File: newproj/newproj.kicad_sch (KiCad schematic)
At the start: 1 part

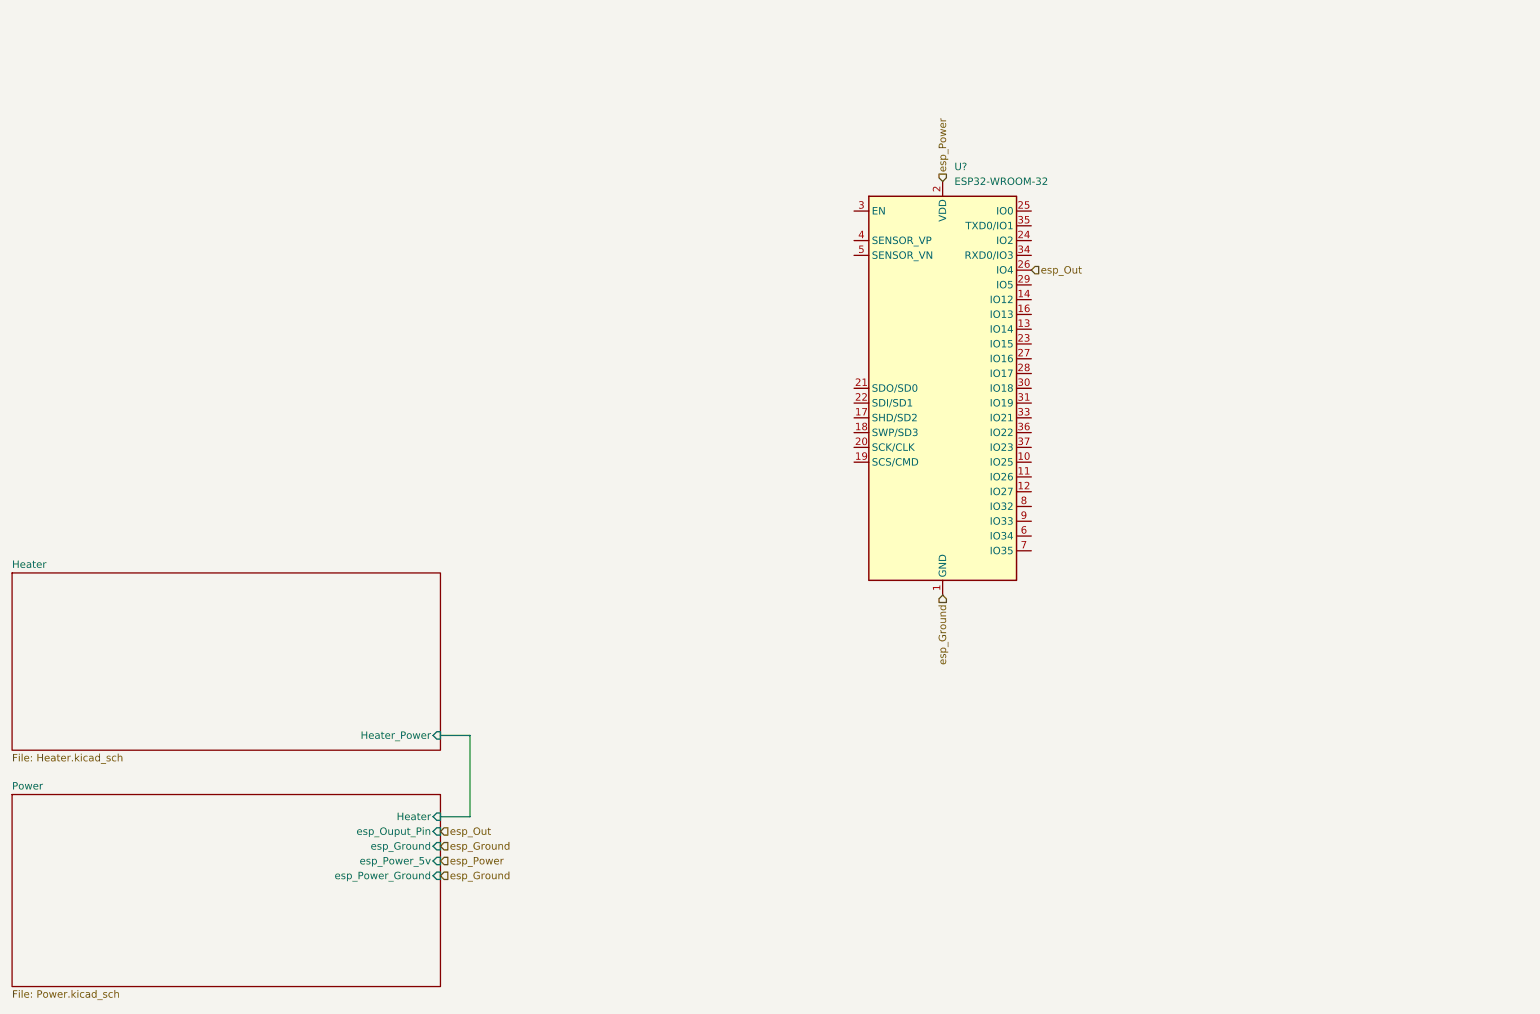
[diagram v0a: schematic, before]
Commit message: Add files via upload
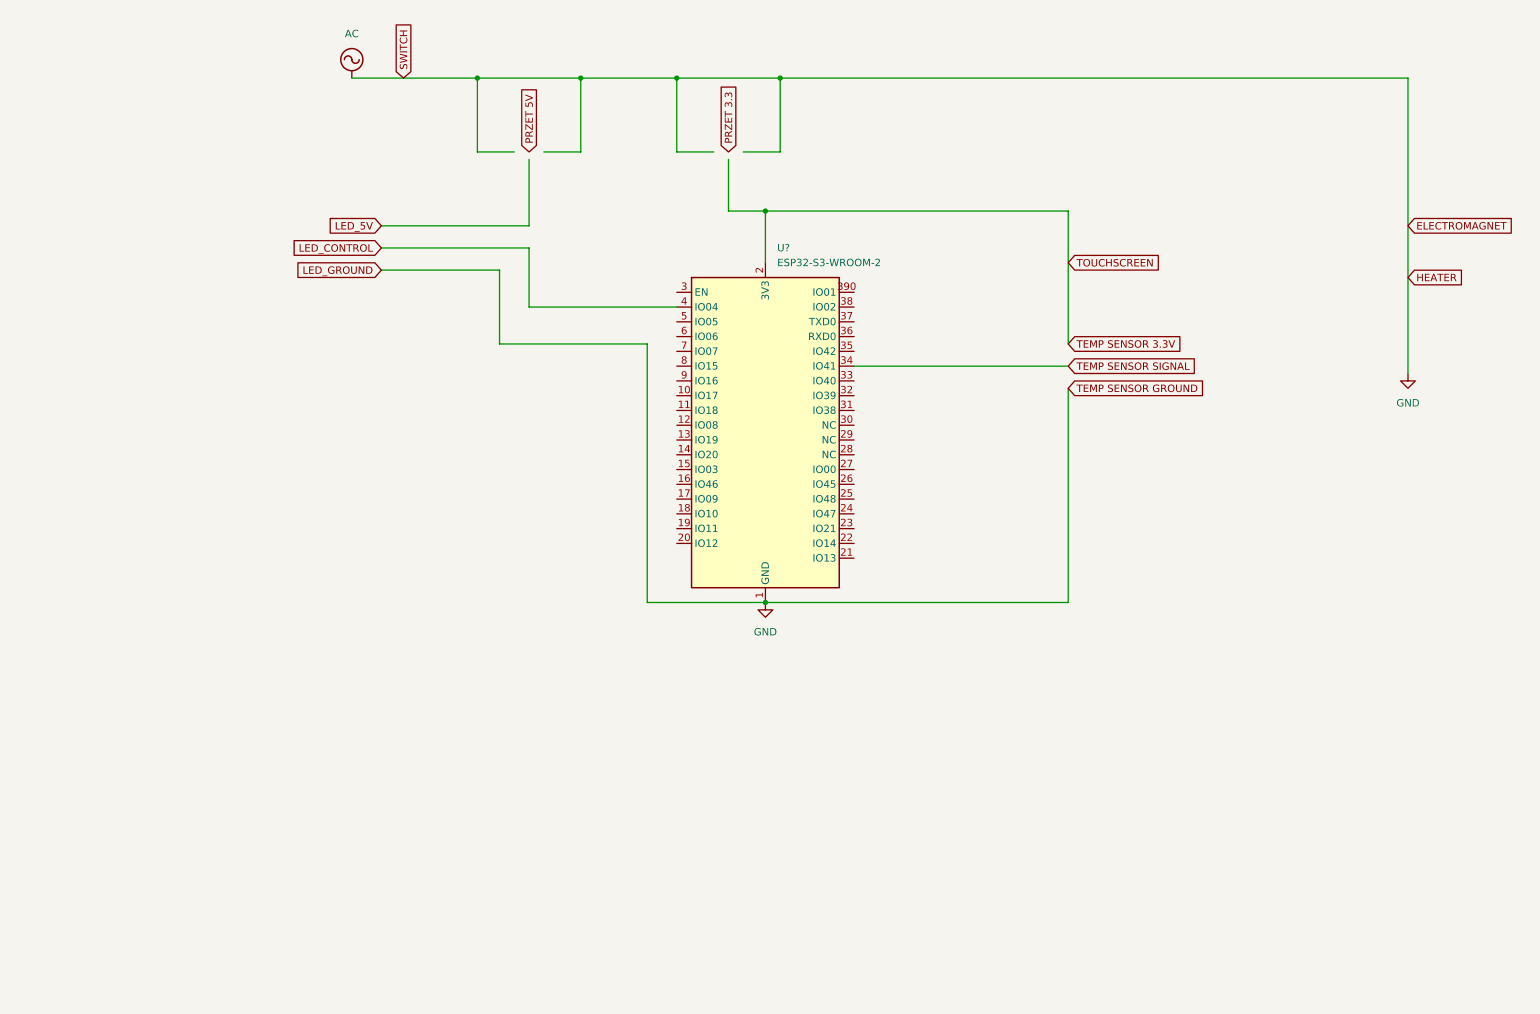
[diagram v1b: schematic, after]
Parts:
- removed U?: ESP32-WROOM-32, RF_Module:ESP32-WROOM-32, symbol RF_Module:ESP32-WROOM-32
- added U?: ESP32-S3-WROOM-2, RF_Module:ESP32-S3-WROOM-2, symbol New_Library:ESP32-S3-WROOM-2
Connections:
- new net AC: U?.1 (GND), U?.26 (IO45), U?.42 (GND), U?.43 (GND)
- new net LED_CONTROL: U?.4 (IO04)
- new net TEMP SENSOR 3.3V: U?.2 (3V3)
- new net TEMP SENSOR SIGNAL: U?.34 (IO41)
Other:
- removed sheet Heater
- removed sheet Power
